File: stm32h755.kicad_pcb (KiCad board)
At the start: 2 copper layers, 80.1 x 49.4 mm, 31 parts, among them U1 STM32H757IITx

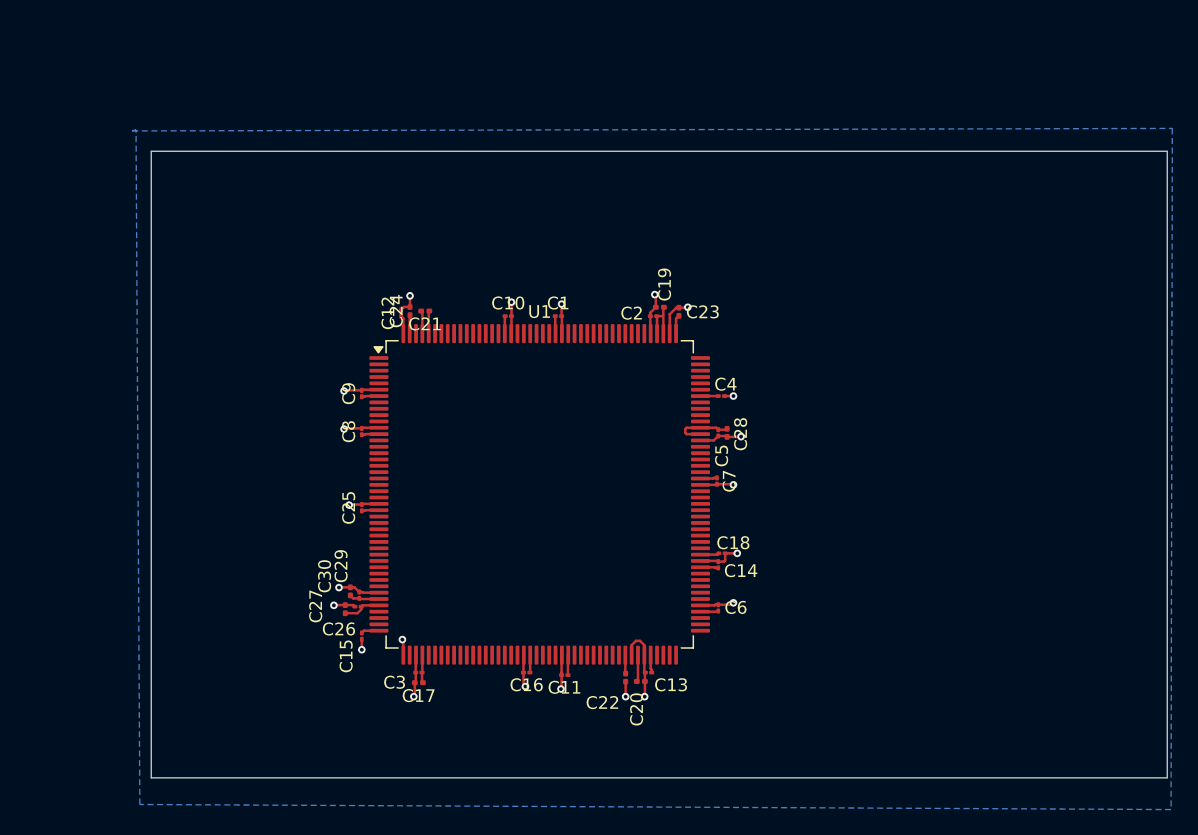
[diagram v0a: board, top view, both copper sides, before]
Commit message: Redesigned PCB
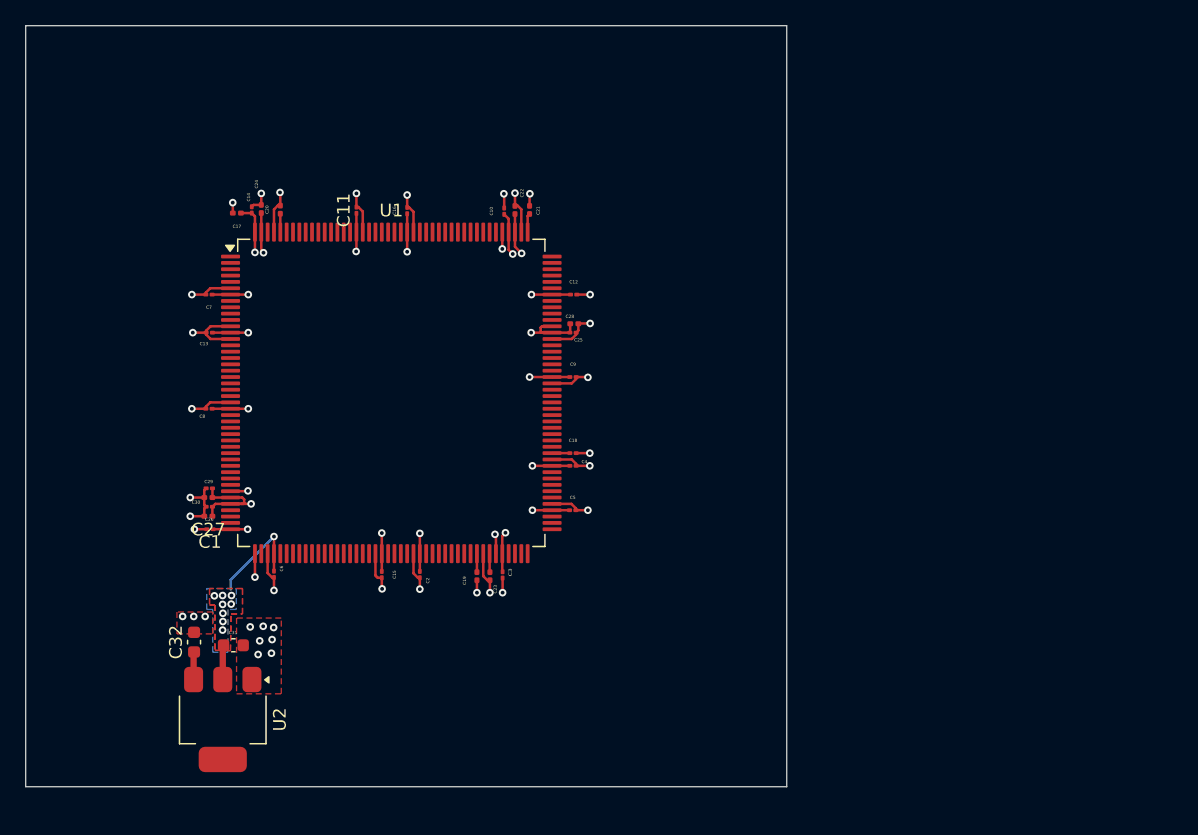
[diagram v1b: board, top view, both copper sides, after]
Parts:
- added C31: 10uF, Capacitor_SMD:C_0603_1608Metric, F.Cu at (86.4, 98.8)
- added C32: 10uF, Capacitor_SMD:C_0603_1608Metric, F.Cu at (83.3, 98.6)
- added U2: AMS1117, Package_TO_SOT_SMD:SOT-223-3_TabPin2, F.Cu at (85.5, 104.7)
- moved C14 46.2 mm to (87.8, 64.5)
- moved C20 45.9 mm to (90.1, 64.5), turned to 90 degrees
- moved C13 43.8 mm to (84.5, 74.2)
- moved C7 42.7 mm to (84.5, 71.2), turned to 180 degrees
- moved C11 40.2 mm to (96.1, 64.5), turned to 90 degrees
- moved C17 39.7 mm to (86.7, 64.8)
- moved C22 38.5 mm to (108.6, 64.5), turned to 90 degrees
- moved C16 37.6 mm to (100.1, 64.6), turned to 90 degrees
- moved C6 35.1 mm to (89.6, 93.2), turned to -90 degrees
- moved C1 32.2 mm to (84.5, 89.7), turned to 180 degrees
- moved C2 27.5 mm to (101.1, 93.3), turned to -90 degrees
- moved C19 26.2 mm to (105.6, 93.4), turned to -90 degrees
- moved C23 25.1 mm to (106.6, 93.4), turned to -90 degrees
- moved C25 21.6 mm to (113.2, 74.2), turned to 0 degrees
- moved C9 16.7 mm to (113.2, 77.7), turned to 0 degrees
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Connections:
- C1 pad 1: +3V3 -> +3.3VA
- C10 pad 1: +3V3 -> +3.3VA
- C11 pad 1: +3V3 -> +3.3VA
- C12 pad 1: +3V3 -> +3.3VA
- C13 pad 1: +3V3 -> +3.3VA
- C14 pad 1: +3V3 -> +3.3VA
- C15 pad 1: +3V3 -> +3.3VA
- C16 pad 1: +3V3 -> +3.3VA
- C17 pad 1: +3V3 -> +3.3VA
- C2 pad 1: +3V3 -> +3.3VA
- C22 pad 1: +3V3 -> +3.3VA
- C23 pad 1: +3V3 -> +3.3VA
- C24 pad 1: +3V3 -> +3.3VA
- C25 pad 1: +3V3 -> +3.3VA
- C28 pad 1: +3V3 -> +3.3VA
- C29 pad 1: /VREF -> +3.3VA
- C3 pad 1: +3V3 -> +3.3VA
- C30 pad 1: /VREF -> +3.3VA
- C4 pad 1: +3V3 -> +3.3VA
- C5 pad 1: +3V3 -> +3.3VA
- C6 pad 1: +3V3 -> +3.3VA
- C7 pad 1: +3V3 -> +3.3VA
- C8 pad 1: +3V3 -> +3.3VA
- C9 pad 1: +3V3 -> +3.3VA
- U1 pad 113: +3V3 -> +3.3VA
- U1 pad 120: +3V3 -> +3.3VA
- U1 pad 121: +3V3 -> +3.3VA
- U1 pad 126: +3V3 -> +3.3VA
- U1 pad 13: +3V3 -> +3.3VA
- U1 pad 135: +3V3 -> +3.3VA
- U1 pad 136: +3V3 -> +3.3VA
- U1 pad 152: +3V3 -> +3.3VA
- U1 pad 160: +3V3 -> +3.3VA
- U1 pad 175: +3V3 -> +3.3VA
- U1 pad 176: +3V3 -> +3.3VA
- U1 pad 25: +3V3 -> +3.3VA
- U1 pad 39: /VREF -> +3.3VA
- U1 pad 44: +3V3 -> +3.3VA
- U1 pad 48: +3V3 -> +3.3VA
- U1 pad 65: +3V3 -> +3.3VA
- U1 pad 7: +3V3 -> +3.3VA
- U1 pad 71: +3V3 -> +3.3VA
- U1 pad 82: +3V3 -> +3.3VA
- U1 pad 84: +3V3 -> +3.3VA
- U1 pad 92: +3V3 -> +3.3VA
- U1 pad 99: +3V3 -> +3.3VA
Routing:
- net +3.3VA: track 3.04 -> 79.0 mm, vias 0 -> 28
- net +3V3: track 34.2 -> 0.00 mm
- net GND: track 58.8 -> 72.5 mm, vias 22 -> 40
- net /VREF: track 2.37 -> 0.00 mm
- net /VIN: track 0.00 -> 2.19 mm
- added copper zone on B.Cu, net +3.3VA
- added copper zone on F.Cu, net +3.3VA
- added copper zone on F.Cu, net GND
- added copper zone on In1.Cu, net GND
- added copper zone on In2.Cu, net GND
- removed copper zone on B.Cu, net GND
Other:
- board size 80.1 x 49.4 mm -> 60 x 60 mm
- copper layers 2 -> 4
